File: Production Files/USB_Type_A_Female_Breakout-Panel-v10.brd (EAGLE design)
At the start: 133.9 x 116.8 mm, 243 parts

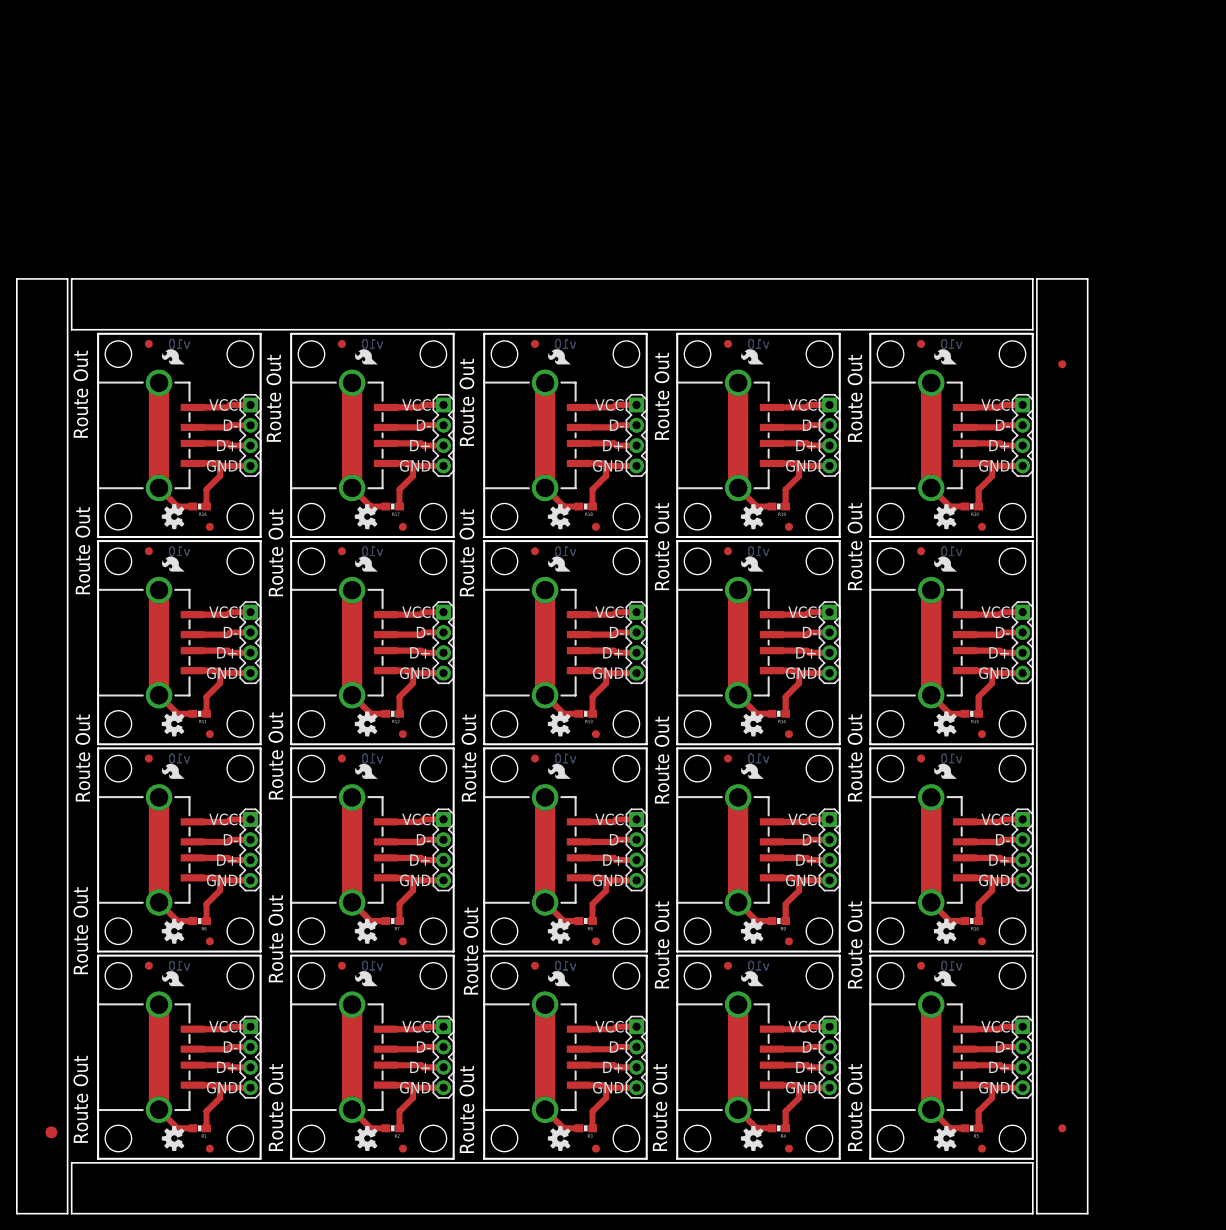
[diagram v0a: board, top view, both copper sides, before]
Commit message: re-did panel v10
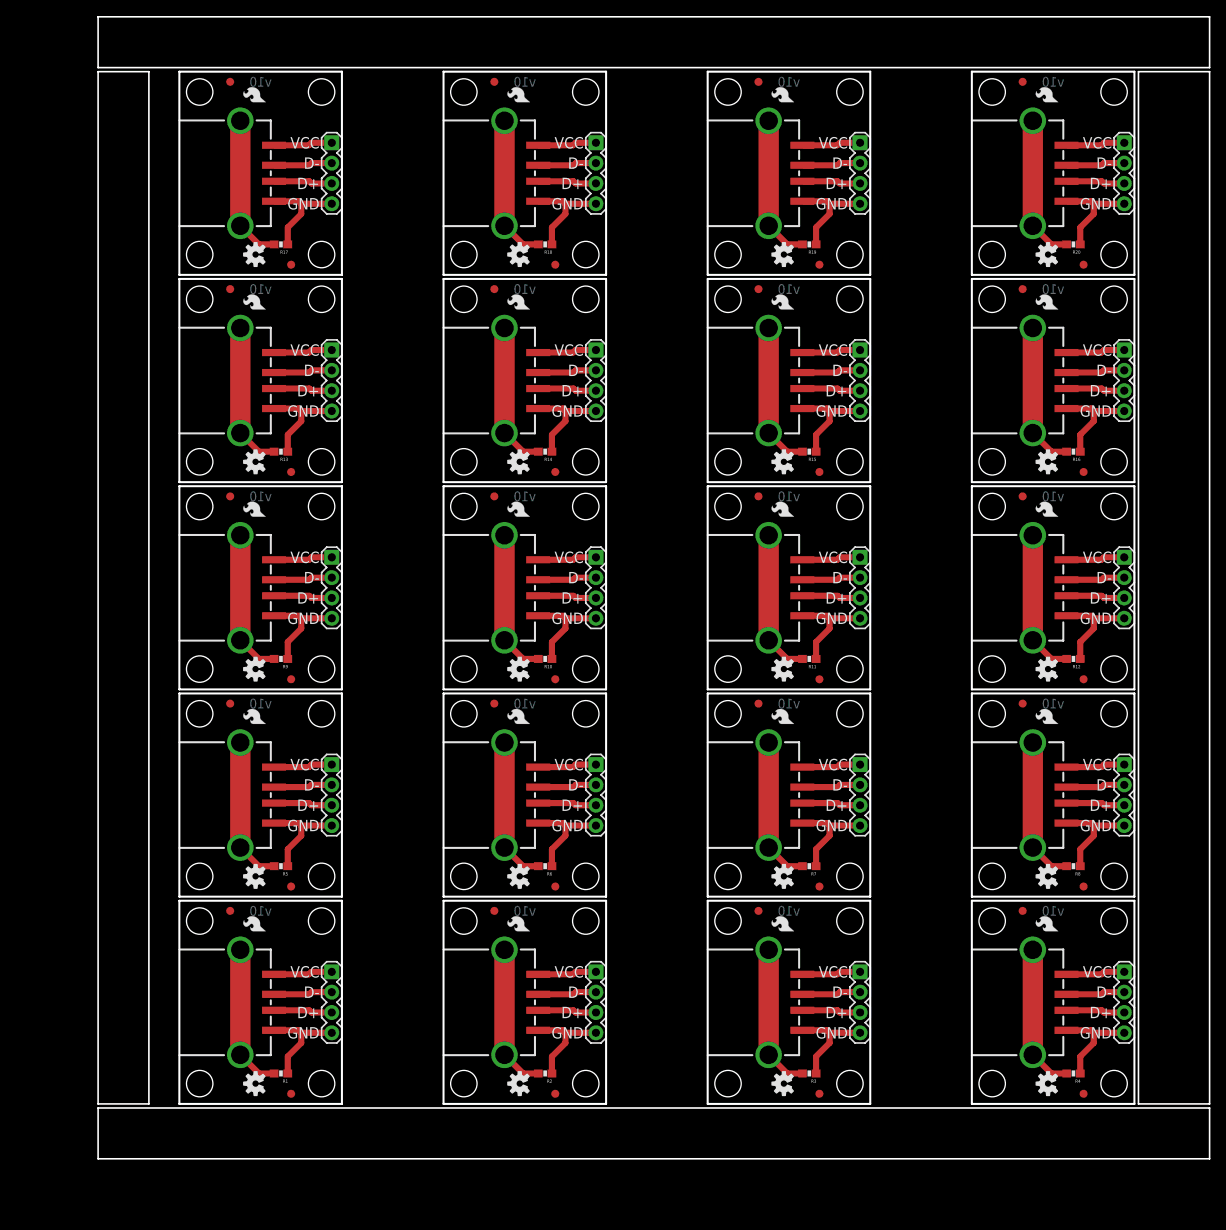
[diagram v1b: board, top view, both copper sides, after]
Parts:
- removed E$1: (no value), SparkFun-Aesthetics:FIDUCIAL-1.5X3
- removed E$5, E$6: (no value), SparkFun-Aesthetics:FIDUCIAL-1X2
- moved JP32 109.4 mm to (128.3, 101.1)
- moved FID31 109.4 mm to (123.2, 85.9)
- moved FID32 109.4 mm to (115.6, 108.7)
- moved JP31 109.4 mm to (116.8, 97.3)
- moved LOGO46 109.4 mm to (121.9, 106.4)
- moved LOGO47 109.4 mm to (118.7, 87.1)
- moved LOGO48 109.4 mm to (120.0, 106.2)
- moved R16 109.4 mm to (121.9, 88.4)
- moved STANDOFF61 109.4 mm to (111.8, 107.4)
- moved STANDOFF62 109.4 mm to (111.8, 87.1)
- moved STANDOFF63 109.4 mm to (127.0, 107.4)
- moved STANDOFF64 109.4 mm to (127.0, 87.1)
- moved FID10 92.4 mm to (16.5, 56.9)
- moved FID9 92.4 mm to (24.1, 34.0)
- moved JP10 92.4 mm to (29.2, 49.3)
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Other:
- board size 133.9 x 116.8 mm -> 138.9 x 142.7 mm
- board text removed: "Route Out"
